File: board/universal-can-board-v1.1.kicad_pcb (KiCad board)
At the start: 2 copper layers, 49.5 x 111.8 mm, 70 parts, among them IC1 ATMEGA328P-A, P1 USB_OTG, P2 CONN_01X08, P3 CONN_01X02, P4 CONN_01X08, P5 CONN_01X08, U1 FT232RL, U2 LM1117-3.3, U3 MCP2515-I/ST, U4 MCP2551-I/SN, Y1 ABM3B_16M, Y2 ABM3B_16M

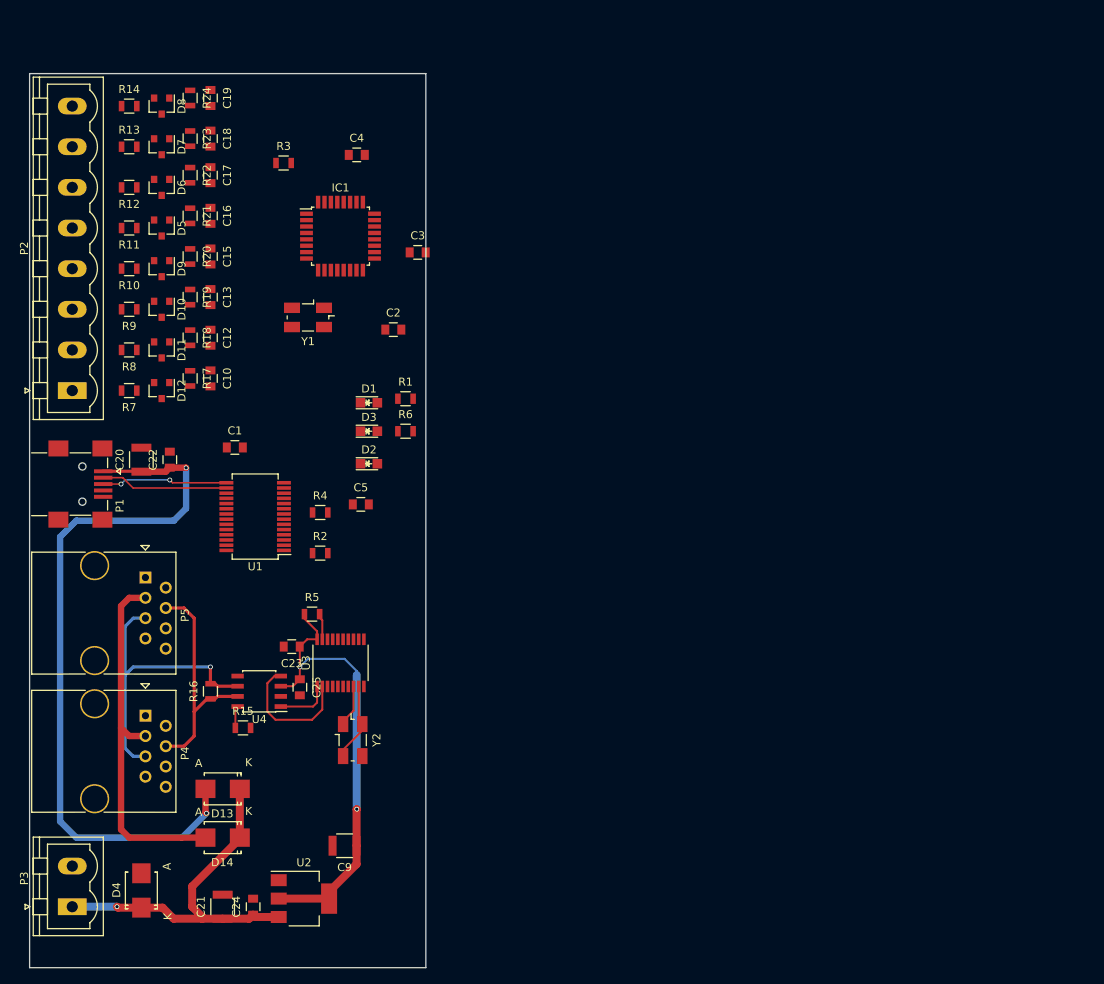
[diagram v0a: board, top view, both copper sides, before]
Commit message: Just saved new pcb layout try.
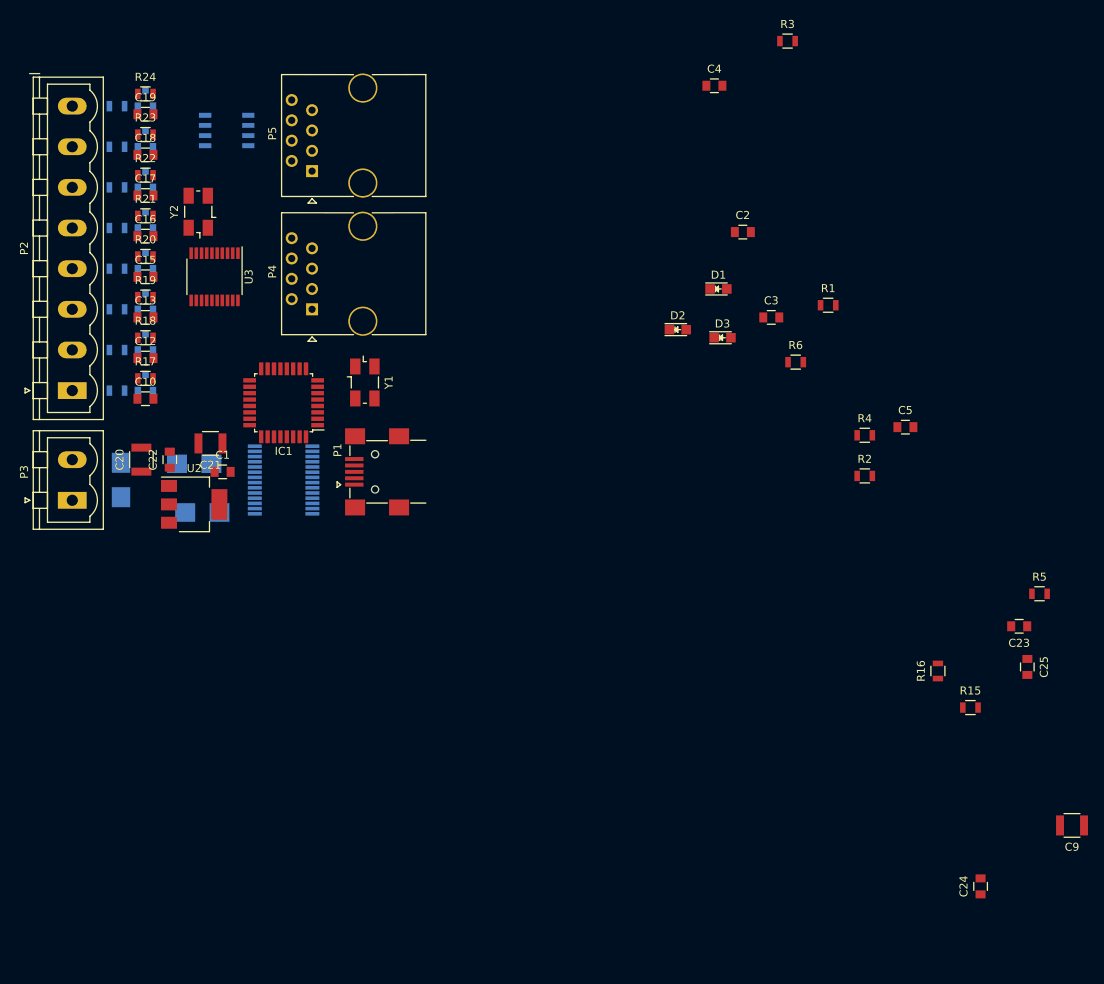
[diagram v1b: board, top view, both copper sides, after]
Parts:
- D10, D11, D12, D13, D14, D4, D5, D6, D7, D8, D9, R10, R11, R12, R13, R14, R7, R8, R9, U1, U4: moved to B.Cu
- moved C23 91.0 mm to (244.3, 119.9)
- moved C25 91.0 mm to (245.4, 125.0)
- moved R15 91.0 mm to (238.3, 130.0)
- moved R5 91.0 mm to (246.9, 115.8)
- moved C24 91.0 mm to (239.5, 152.4)
- moved C9 91.0 mm to (251.0, 144.8)
- moved R16 91.0 mm to (234.2, 125.5)
- moved U4 70.2 mm to (145.3, 57.9), turned to 0 degrees
- moved Y2 68.8 mm to (141.7, 68.1), turned to 90 degrees
- moved C5 68.8 mm to (230.1, 95.0)
- moved R2 68.8 mm to (225.0, 101.1)
- moved R4 68.8 mm to (225.0, 96.0)
- moved R3 64.8 mm to (215.4, 46.7)
- moved C21 57.9 mm to (143.3, 97.0), turned to 180 degrees
- moved P4 54.9 mm to (156.0, 80.3), turned to 90 degrees
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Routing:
- net Net-(C20-Pad1): track 92.5 -> 0.00 mm, vias 2 -> 0
- net VCC: track 57.5 -> 0.00 mm, vias 2 -> 0
- net +5V: track 46.3 -> 0.00 mm, vias 1 -> 0
- net Net-(D14-Pad2): track 45.8 -> 0.00 mm
- net Net-(P4-Pad5): track 37.9 -> 0.00 mm, vias 1 -> 0
- net Net-(P4-Pad4): track 29.1 -> 0.00 mm
- net Net-(U3-Pad2): track 16.3 -> 0.00 mm
- net USB_D-: track 15.9 -> 0.00 mm
- net USB_D+: track 15.7 -> 0.00 mm, vias 2 -> 0
- net Net-(U3-Pad9): track 10.9 -> 0.00 mm
- net Net-(U3-Pad1): track 6.75 -> 0.00 mm
- net Net-(U3-Pad8): track 5.24 -> 0.00 mm
- net RESET: track 3.28 -> 0.00 mm
- net Net-(R15-Pad1): track 2.78 -> 0.00 mm
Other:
- board outline removed

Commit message: Moved on with the layout.
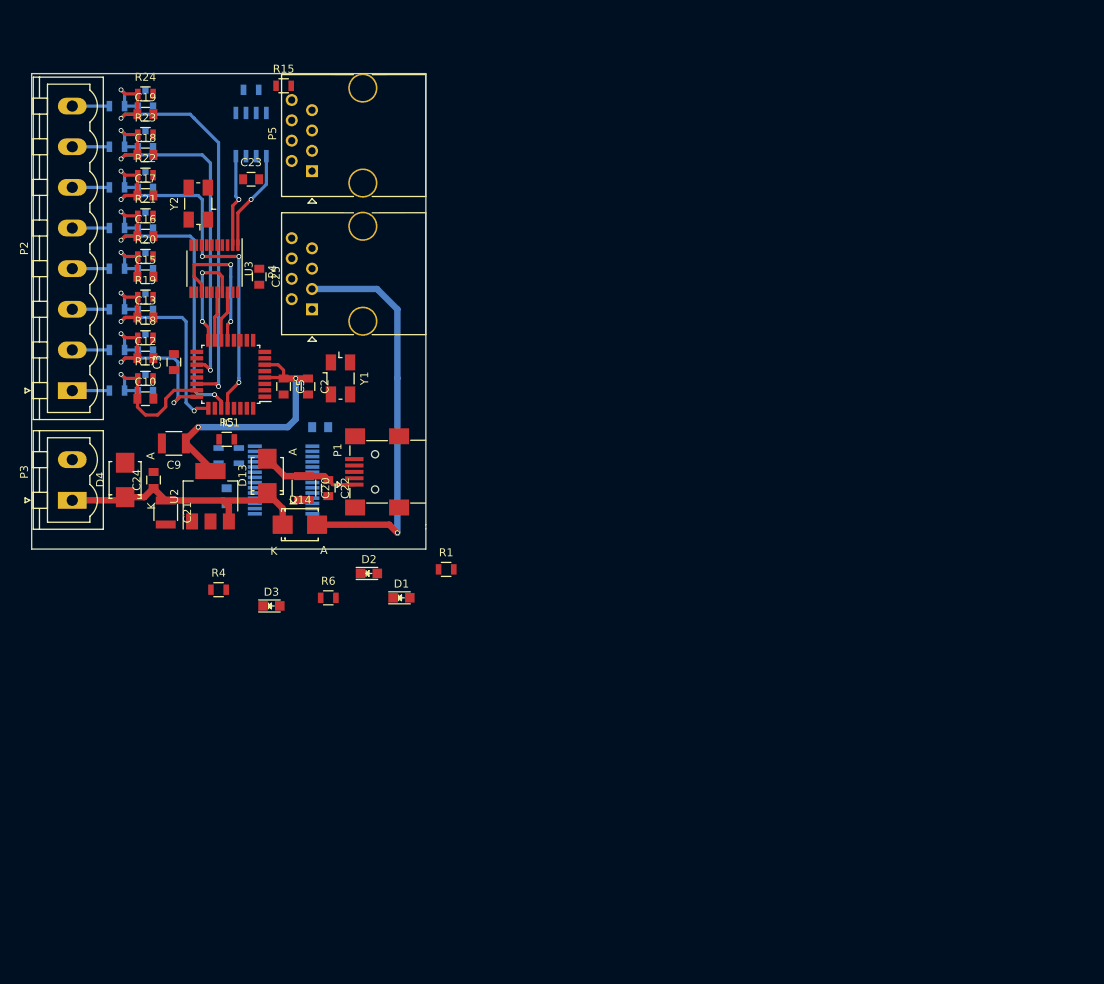
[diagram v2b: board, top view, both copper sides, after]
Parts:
- C1, C4, R16, R2, R3: moved to B.Cu
- D13, D14, D4: moved to F.Cu
- moved C9 122.0 mm to (138.7, 97.0)
- moved R15 115.8 mm to (152.4, 52.3)
- moved C24 115.2 mm to (136.1, 101.6)
- moved R16 112.5 mm to (148.3, 52.8), turned to 180 degrees
- moved C23 111.1 mm to (148.3, 64.0), turned to 0 degrees
- moved C25 107.7 mm to (149.4, 76.2)
- moved R5 103.4 mm to (145.3, 96.5)
- moved R3 88.0 mm to (144.3, 98.6), turned to 90 degrees
- moved R4 83.0 mm to (144.3, 115.3)
- moved C4 79.7 mm to (145.3, 103.6), turned to 270 degrees
- moved R2 78.3 mm to (146.8, 98.6), turned to 270 degrees
- moved C5 77.9 mm to (152.4, 89.9), turned to 270 degrees
- moved C3 74.9 mm to (138.7, 86.9), turned to 90 degrees
- moved D3 65.6 mm to (150.9, 117.3)
- moved R6 65.4 mm to (158.0, 116.3)
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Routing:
- net IO7: track 0.00 -> 58.2 mm, vias 0 -> 3
- net IO5: track 0.00 -> 52.8 mm, vias 0 -> 5
- net IO6: track 0.00 -> 50.7 mm, vias 0 -> 3
- net Net-(D14-Pad2): track 0.00 -> 50.1 mm, vias 0 -> 1
- net IO4: track 0.00 -> 44.2 mm, vias 0 -> 3
- net VCC: track 0.00 -> 34.2 mm, vias 0 -> 2
- net +5V: track 0.00 -> 33.8 mm
- net IO2: track 0.00 -> 33.1 mm, vias 0 -> 3
- net IO1: track 0.00 -> 27.0 mm, vias 0 -> 3
- net IO0: track 0.00 -> 19.5 mm, vias 0 -> 1
- net CAN_INT: track 0.00 -> 18.0 mm, vias 0 -> 2
- net CAN_SO: track 0.00 -> 13.4 mm, vias 0 -> 2
- net Net-(U3-Pad1): track 0.00 -> 12.6 mm, vias 0 -> 1
- net Net-(C20-Pad1): track 0.00 -> 12.2 mm
- net Net-(U3-Pad2): track 0.00 -> 11.6 mm, vias 0 -> 1
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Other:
- board outline added: 49.3 x 59.4 mm
